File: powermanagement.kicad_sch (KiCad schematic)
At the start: 35 parts, among them J9 Battery, Q2 AP2302B, SW6 SW_SPDT, U4 TPS63020DSJR, U5 XT4054K421MR-G, U6 SY6280AAC

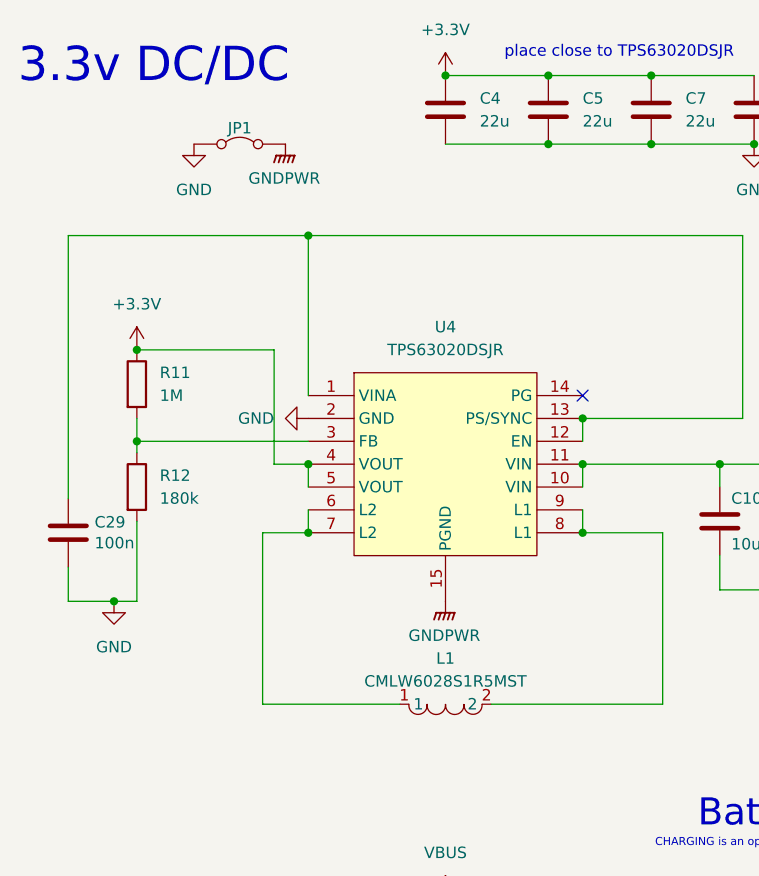
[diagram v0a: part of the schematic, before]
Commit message: Changes for production version
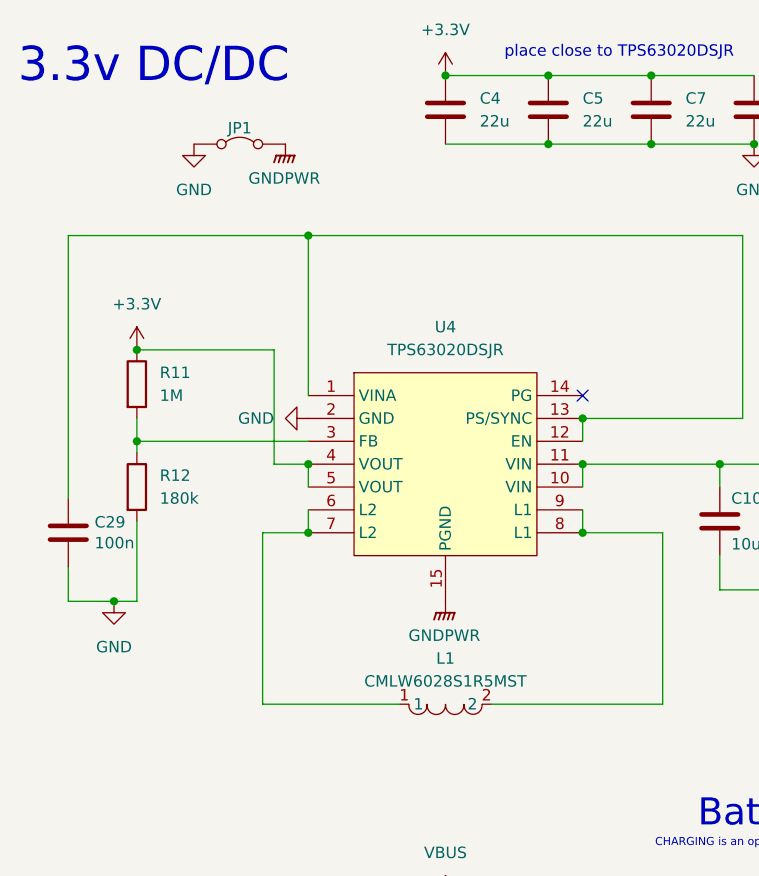
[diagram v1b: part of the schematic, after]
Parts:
- U6: footprint library:SOT-23-5 -> Package_TO_SOT_SMD:SOT-23-5
